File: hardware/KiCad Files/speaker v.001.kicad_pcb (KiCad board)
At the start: 2 copper layers, 40 x 30 mm, 14 parts, among them U1 LM386N

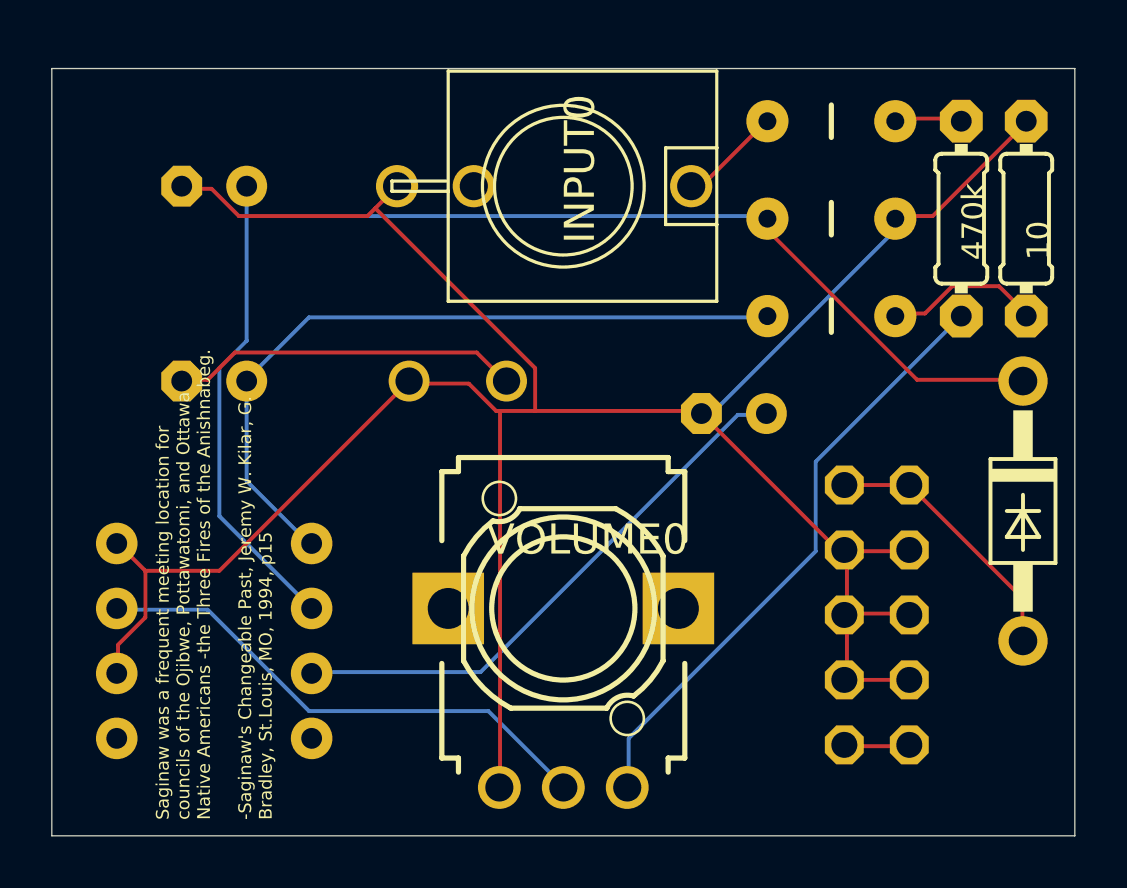
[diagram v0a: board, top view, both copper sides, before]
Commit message: Updated PCB design
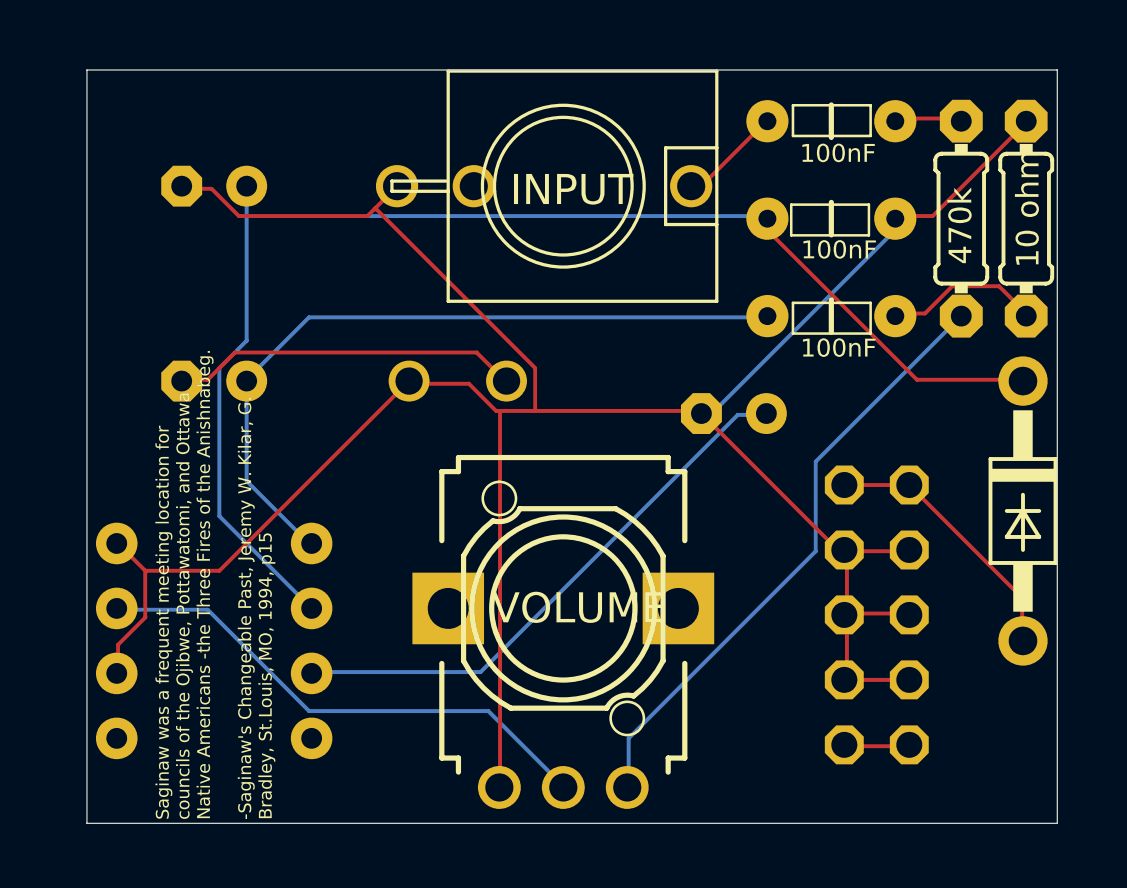
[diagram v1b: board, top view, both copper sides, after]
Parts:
- R1: value 10 -> 10 ohm
- renumbered INPUT0 to INPUT, VOLUME0 to VOLUME
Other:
- board size 40 x 30 mm -> 37.9 x 29.5 mm
- board text added: "Saginaw Speaker v002 JUL 2021 North Coast Modular Collective"
- board text removed: "Saginaw Speaker v001 JUL 2021 North Coast Modular Collective"
